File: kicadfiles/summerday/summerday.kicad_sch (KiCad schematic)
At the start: 106 parts, among them J1 USB_C_Receptacle_USB2.0_14P, SW1 SW_DPST_x2, SW2 SW_DPST_x2, U1 XC6206PxxxMR, U2 STM32F072CBTx, U3 SRV05-4

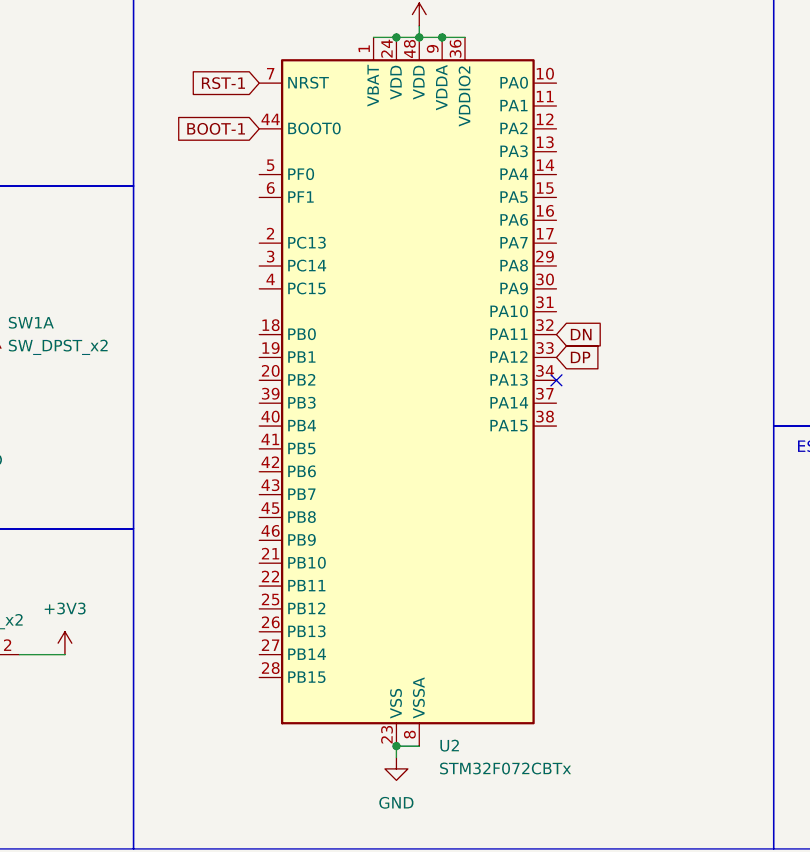
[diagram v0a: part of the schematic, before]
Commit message: Almost Finished pcb artworks
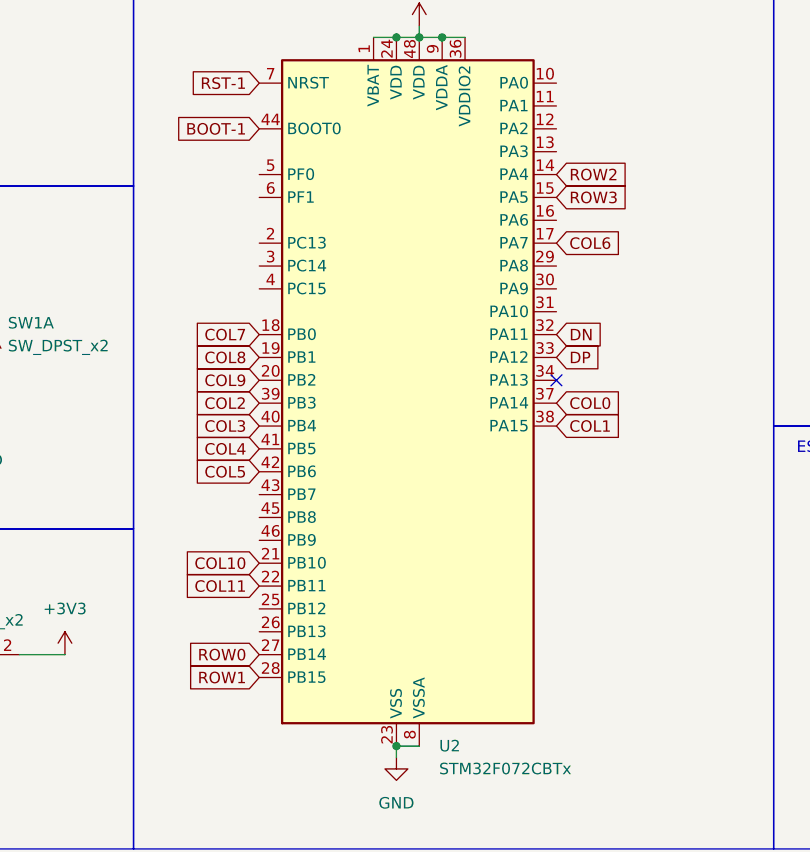
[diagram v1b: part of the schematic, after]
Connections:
- net COL0: now also U2.37 (PA14)
- net COL1: now also U2.38 (PA15)
- net COL10: now also U2.21 (PB10)
- net COL11: now also U2.22 (PB11)
- net COL2: now also U2.39 (PB3)
- net COL3: now also U2.40 (PB4)
- net COL4: now also U2.41 (PB5)
- net COL5: now also U2.42 (PB6)
- net COL6: now also U2.17 (PA7)
- net COL7: now also U2.18 (PB0)
- net COL8: now also U2.19 (PB1)
- net COL9: now also U2.20 (PB2)
- net ROW0: now also U2.27 (PB14)
- net ROW1: now also U2.28 (PB15)
- net ROW2: now also U2.14 (PA4)
- net ROW3: now also U2.15 (PA5)
